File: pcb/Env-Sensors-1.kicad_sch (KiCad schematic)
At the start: 15 parts, among them J1 SEN66, U10 SCD41, U14 SHT45, U9 SGP41

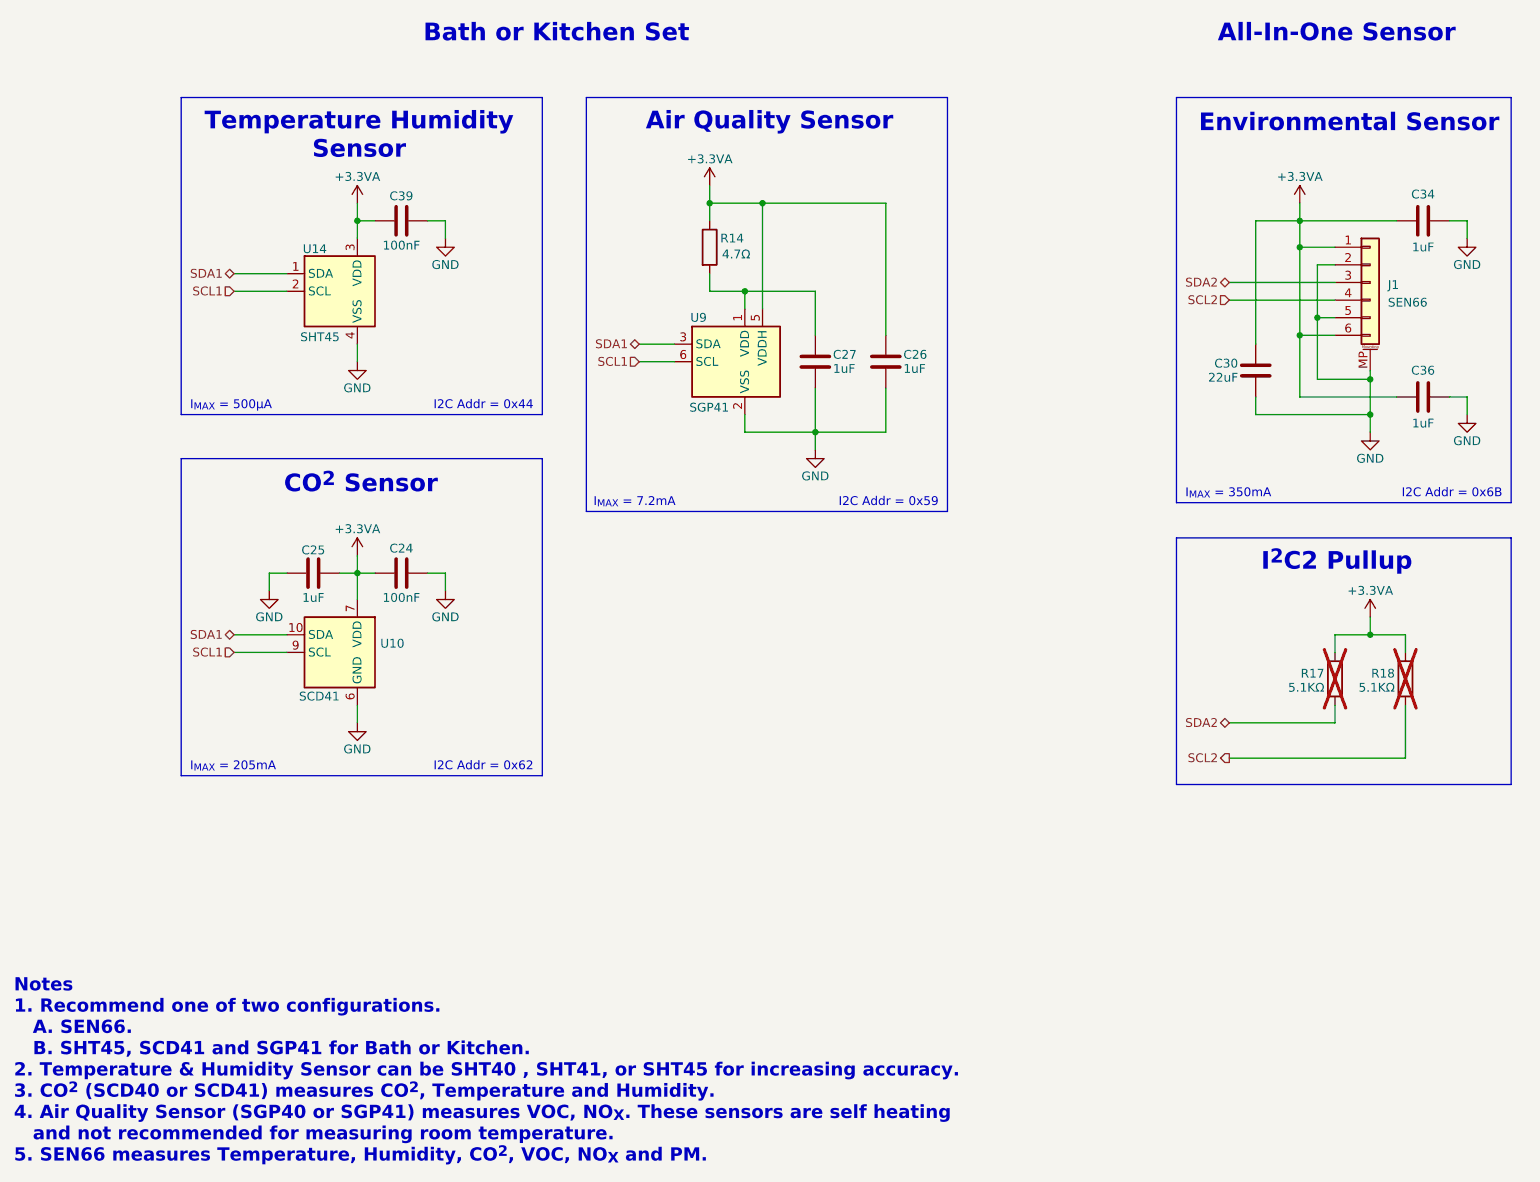
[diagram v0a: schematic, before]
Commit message: Cleanup schematic, BOM and update gerber files
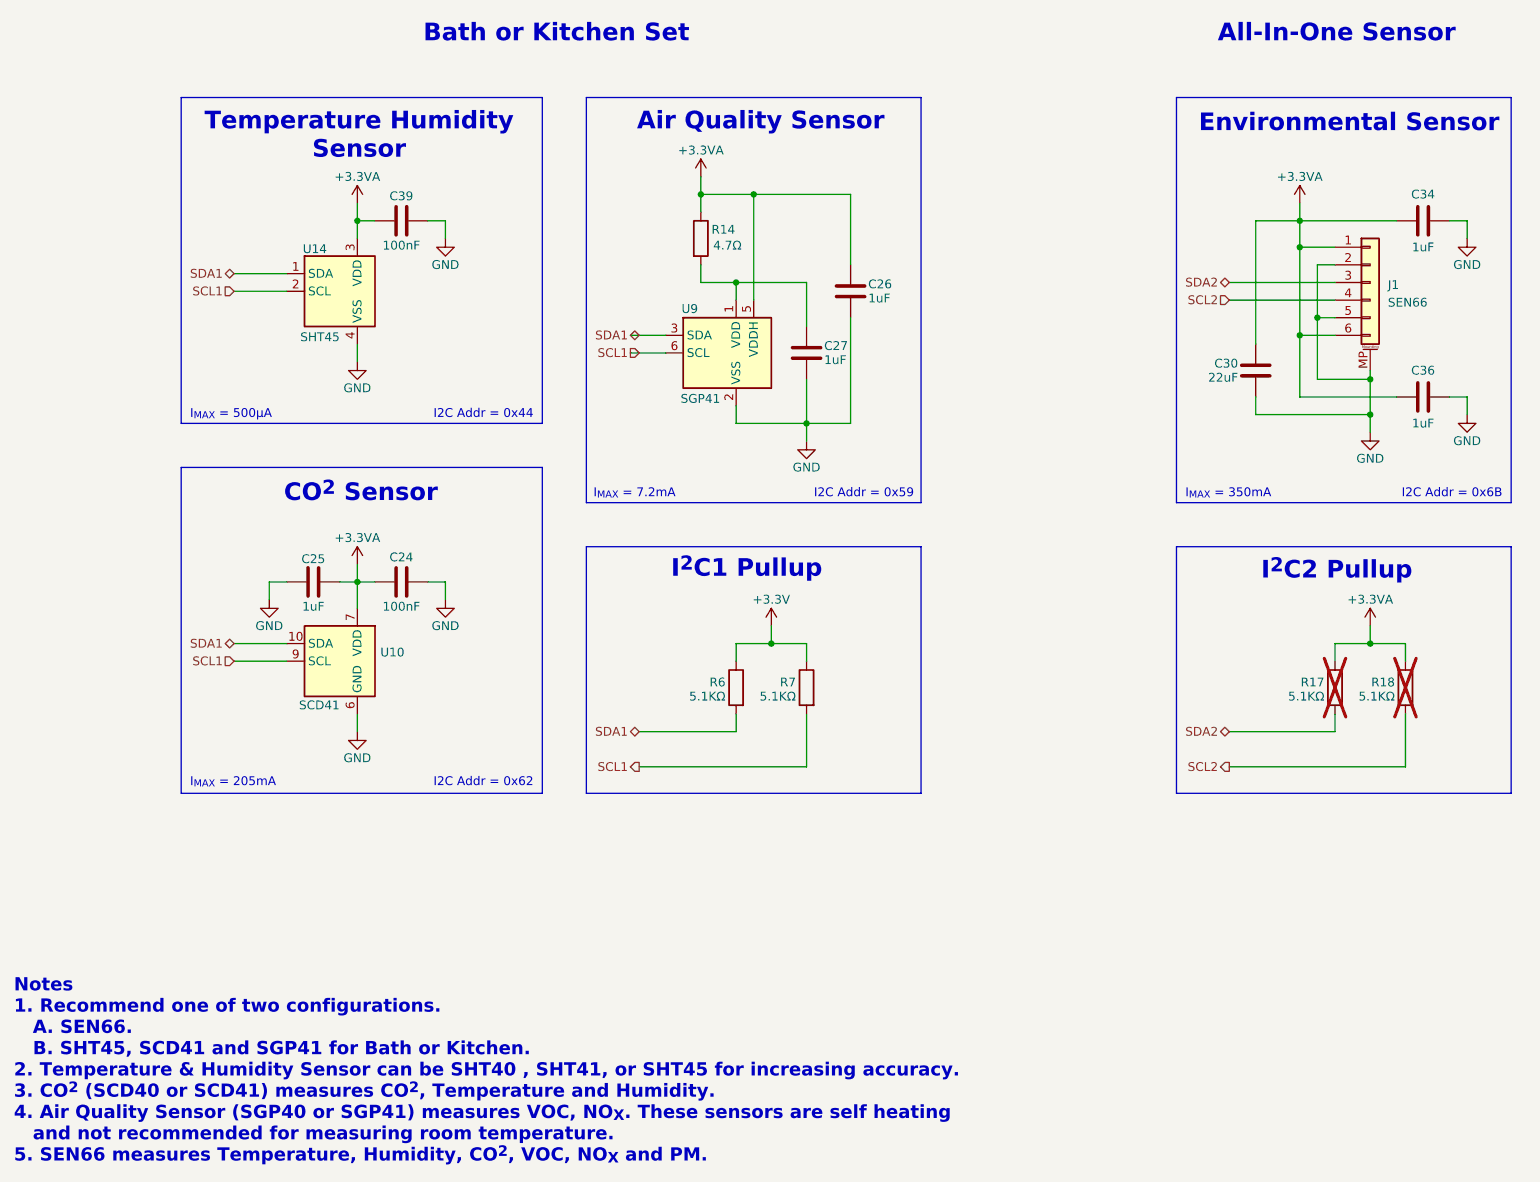
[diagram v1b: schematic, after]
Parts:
- added R6, R7: 5.1KΩ, Resistor_SMD:R_0402_1005Metric, symbol Device:R
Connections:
- net SCL1: now also R7.2
- net SDA1: now also R6.2
- new net +3.3V: R6.1, R7.1
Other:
- note added: "I^{2}C1 Pullup"
- moved on the sheet: C24, C25, C26, C27, R14, R17, R18, U10, U9
